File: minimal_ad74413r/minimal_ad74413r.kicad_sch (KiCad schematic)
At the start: 60 parts, among them J1 FW-02-03-G-D-085-155, J2 FW-02-03-G-D-085-155, J3 FW-02-03-G-D-085-155, J4 FW-02-03-G-D-085-155, J5 FW-02-03-G-D-085-155, J6 FW-02-03-G-D-085-155, J7 FW-14-03-G-D-085-155, U1 AD74413RBCPZ

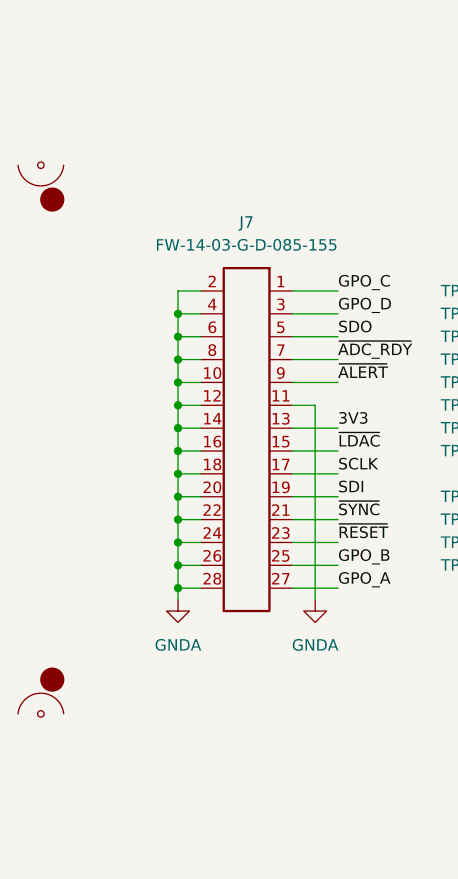
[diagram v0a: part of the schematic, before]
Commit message: Development backup
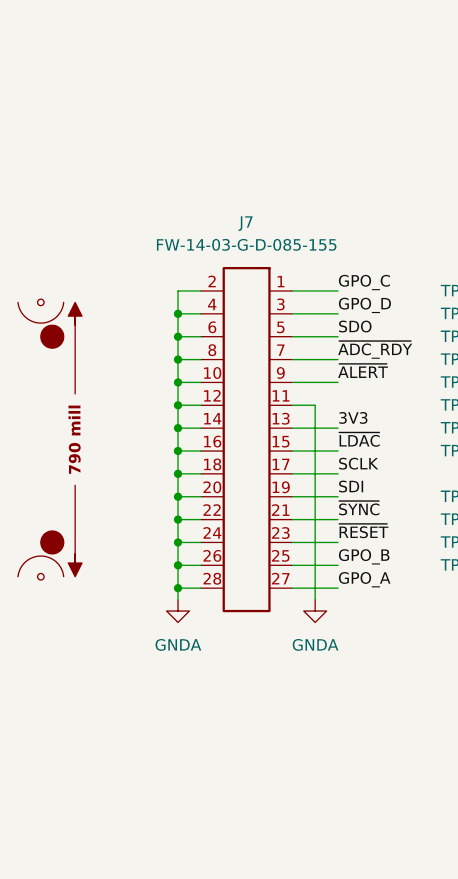
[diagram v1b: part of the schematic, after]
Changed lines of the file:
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@@
 		(dnp no)
 		(fields_autoplaced yes)
-		(property "Reference" "#PWR7"
+		(property "Reference" "#PWR11"
 			(at 233.68 68.58 0)
 			(effects
@@
 			(project "minimal_ad74413r"
 				(path "/3d1a8eae-9f4e-4ae3-8a80-a6e3408e9f8d"
-					(reference "#PWR7")
+					(reference "#PWR11")
 					(unit 1)
 				)
@@
 		(dnp no)
 		(fields_autoplaced yes)
-		(property "Reference" "#PWR22"
+		(property "Reference" "#PWR3"
 			(at 162.56 74.93 0)
 			(effects
@@
 			(project "minimal_ad74413r"
 				(path "/3d1a8eae-9f4e-4ae3-8a80-a6e3408e9f8d"
-					(reference "#PWR22")
+					(reference "#PWR3")
 					(unit 1)
 				)
@@
 		(dnp no)
 		(fields_autoplaced yes)
-		(property "Reference" "#PWR29"
+		(property "Reference" "#PWR2"
 			(at 137.16 187.96 0)
 			(effects
@@
 			(project "minimal_ad74413r"
 				(path "/3d1a8eae-9f4e-4ae3-8a80-a6e3408e9f8d"
-					(reference "#PWR29")
+					(reference "#PWR2")
 					(unit 1)
 				)
@@
 		(dnp no)
 		(fields_autoplaced yes)
-		(property "Reference" "#PWR6"
+		(property "Reference" "#PWR10"
 			(at 228.6 52.07 0)
 			(effects
@@
 			(project "minimal_ad74413r"
 				(path "/3d1a8eae-9f4e-4ae3-8a80-a6e3408e9f8d"
-					(reference "#PWR6")
+					(reference "#PWR10")
 					(unit 1)
 				)
@@
 		(dnp no)
 		(fields_autoplaced yes)
-		(property "Reference" "#PWR32"
+		(property "Reference" "#PWR15"
 			(at 284.48 137.16 0)
 			(effects
@@
 			(project "minimal_ad74413r"
 				(path "/3d1a8eae-9f4e-4ae3-8a80-a6e3408e9f8d"
-					(reference "#PWR32")
+					(reference "#PWR15")
 					(unit 1)
 				)
@@
 		(dnp no)
 		(fields_autoplaced yes)
-		(property "Reference" "#PWR9"
+		(property "Reference" "#PWR14"
 			(at 243.84 104.14 0)
 			(effects
@@
 			(project "minimal_ad74413r"
 				(path "/3d1a8eae-9f4e-4ae3-8a80-a6e3408e9f8d"
-					(reference "#PWR9")
+					(reference "#PWR14")
 					(unit 1)
 				)
@@
 		(dnp no)
 		(fields_autoplaced yes)
-		(property "Reference" "#PWR36"
+		(property "Reference" "#PWR18"
 			(at 284.48 220.98 0)
 			(effects
@@
 			(project "minimal_ad74413r"
 				(path "/3d1a8eae-9f4e-4ae3-8a80-a6e3408e9f8d"
-					(reference "#PWR36")
+					(reference "#PWR18")
 					(unit 1)
 				)
@@
 		(dnp no)
 		(fields_autoplaced yes)
-		(property "Reference" "#PWR33"
+		(property "Reference" "#PWR16"
 			(at 284.48 165.1 0)
 			(effects
@@
 			(project "minimal_ad74413r"
 				(path "/3d1a8eae-9f4e-4ae3-8a80-a6e3408e9f8d"
-					(reference "#PWR33")
+					(reference "#PWR16")
 					(unit 1)
 				)
@@
 		(dnp no)
 		(fields_autoplaced yes)
-		(property "Reference" "#PWR30"
+		(property "Reference" "#PWR1"
 			(at 121.92 187.96 0)
 			(effects
@@
 			(project "minimal_ad74413r"
 				(path "/3d1a8eae-9f4e-4ae3-8a80-a6e3408e9f8d"
-					(reference "#PWR30")
+					(reference "#PWR1")
 					(unit 1)
 				)
@@
 		(dnp no)
 		(fields_autoplaced yes)
-		(property "Reference" "#PWR4"
+		(property "Reference" "#PWR8"
 			(at 175.26 52.07 0)
 			(effects
@@
 			(project "minimal_ad74413r"
 				(path "/3d1a8eae-9f4e-4ae3-8a80-a6e3408e9f8d"
-					(reference "#PWR4")
+					(reference "#PWR8")
 					(unit 1)
 				)
@@
 		(dnp no)
 		(fields_autoplaced yes)
-		(property "Reference" "#PWR2"
+		(property "Reference" "#PWR7"
 			(at 170.18 219.71 0)
 			(effects
@@
 			(project "minimal_ad74413r"
 				(path "/3d1a8eae-9f4e-4ae3-8a80-a6e3408e9f8d"
-					(reference "#PWR2")
+					(reference "#PWR7")
 					(unit 1)
 				)
@@
 		(dnp no)
 		(fields_autoplaced yes)
-		(property "Reference" "#PWR3"
+		(property "Reference" "#PWR6"
 			(at 167.64 109.22 0)
 			(effects
@@
 			(project "minimal_ad74413r"
 				(path "/3d1a8eae-9f4e-4ae3-8a80-a6e3408e9f8d"
-					(reference "#PWR3")
+					(reference "#PWR6")
 					(unit 1)
 				)
@@
 		(dnp no)
 		(fields_autoplaced yes)
-		(property "Reference" "#PWR8"
+		(property "Reference" "#PWR12"
 			(at 238.76 86.36 0)
 			(effects
@@
 			(project "minimal_ad74413r"
 				(path "/3d1a8eae-9f4e-4ae3-8a80-a6e3408e9f8d"
-					(reference "#PWR8")
+					(reference "#PWR12")
 					(unit 1)
 				)
@@
 		(dnp no)
 		(fields_autoplaced yes)
-		(property "Reference" "#PWR1"
+		(property "Reference" "#PWR4"
 			(at 162.56 87.63 0)
 			(effects
@@
 			(project "minimal_ad74413r"
 				(path "/3d1a8eae-9f4e-4ae3-8a80-a6e3408e9f8d"
-					(reference "#PWR1")
+					(reference "#PWR4")
 					(unit 1)
 				)
@@
 		(on_board yes)
 		(dnp no)
-		(property "Reference" "#PWR28"
+		(property "Reference" "#PWR5"
 			(at 167.64 45.72 0)
 			(effects
@@
 			(project "minimal_ad74413r"
 				(path "/3d1a8eae-9f4e-4ae3-8a80-a6e3408e9f8d"
-					(reference "#PWR28")
+					(reference "#PWR5")
 					(unit 1)
 				)
@@
 		(dnp no)
 		(fields_autoplaced yes)
-		(property "Reference" "#PWR5"
+		(property "Reference" "#PWR9"
 			(at 203.2 243.84 0)
 			(effects
@@
 			(project "minimal_ad74413r"
 				(path "/3d1a8eae-9f4e-4ae3-8a80-a6e3408e9f8d"
-					(reference "#PWR5")
+					(reference "#PWR9")
 					(unit 1)
 				)
@@
 		(dnp no)
 		(fields_autoplaced yes)
-		(property "Reference" "#PWR34"
+		(property "Reference" "#PWR17"
 			(at 284.48 193.04 0)
 			(effects
@@
 			(project "minimal_ad74413r"
 				(path "/3d1a8eae-9f4e-4ae3-8a80-a6e3408e9f8d"
-					(reference "#PWR34")
+					(reference "#PWR17")
 					(unit 1)
 				)
@@
 		(on_board yes)
 		(dnp no)
-		(property "Reference" "#PWR27"
+		(property "Reference" "#PWR13"
 			(at 241.3 45.72 0)
 			(effects
@@
 			(project "minimal_ad74413r"
 				(path "/3d1a8eae-9f4e-4ae3-8a80-a6e3408e9f8d"
-					(reference "#PWR27")
+					(reference "#PWR13")
 					(unit 1)
 				)
